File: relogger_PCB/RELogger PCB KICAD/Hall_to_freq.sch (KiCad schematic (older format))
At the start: 12 parts, among them U6 LM393

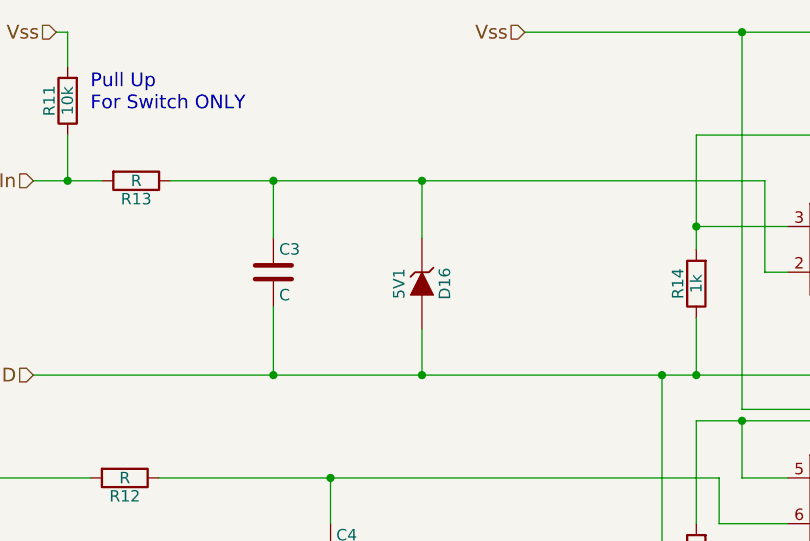
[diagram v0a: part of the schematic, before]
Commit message: Small updates
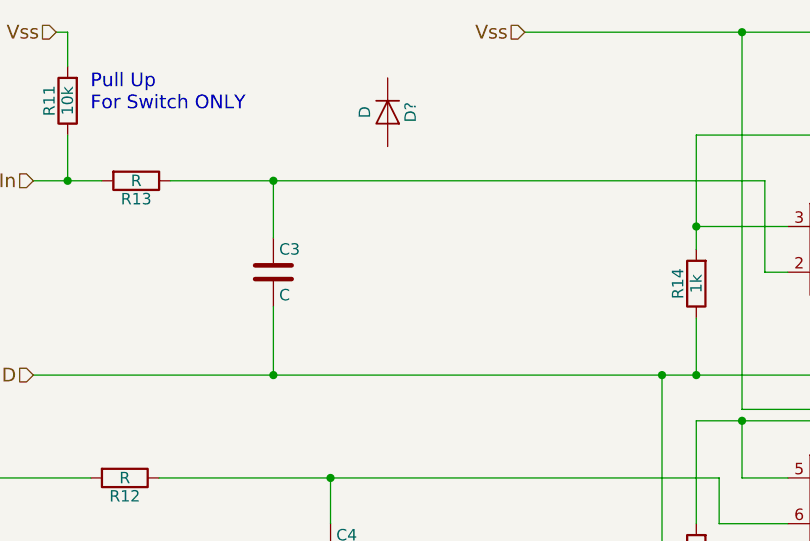
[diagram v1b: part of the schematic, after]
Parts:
- removed D16: 5V1, REInnovationFootprint:TH_Diode_1, symbol ZENER-RESCUE-RELogger_PCB_v1
- added D?: D, symbol D
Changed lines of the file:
@@
 Wire Wire Line
 	7000 3250 7450 3250
-$Comp
-L ZENER-RESCUE-RELogger_PCB_v1 D16
-U 1 1 57B7AFA3
-P 4800 3400
-F 0 "D16" H 4800 3500 50  0000 C CNN
-F 1 "5V1" H 4800 3300 50  0000 C CNN
-F 2 "REInnovationFootprint:TH_Diode_1" H 4800 3400 50  0001 C CNN
-F 3 "" H 4800 3400 50  0000 C CNN
-	1    4800 3400
-	0    1    1    0
-$EndComp
-Wire Wire Line
-	4800 2950 4800 3200
-Connection ~ 4800 2950
-Wire Wire Line
-	4800 3800 4800 3600
-Connection ~ 4800 3800
 Text HLabel 1450 4250 0    60   Input ~ 0
 Freq_IN
@@
 	6200 4250 6200 4000
 Connection ~ 6200 4000
+$Comp
+L D D?
+U 1 1 595D9167
+P 4650 2650
+F 0 "D?" H 4650 2750 50  0000 C CNN
+F 1 "D" H 4650 2550 50  0000 C CNN
+F 2 "" H 4650 2650 50  0000 C CNN
+F 3 "" H 4650 2650 50  0000 C CNN
+	1    4650 2650
+	0    1    1    0
+$EndComp
 $EndSCHEMATC
